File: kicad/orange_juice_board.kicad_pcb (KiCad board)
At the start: 2 copper layers, 85 x 56 mm, 56 parts, among them J10 GPIO12_Head, J10 PWM_OUT1, J11 CONN_UART, J12 Conn_01x08, J12 PWM_OUT2, J13 GPIO6_Head, J14 GPIO11_Head, J15 PWM_OUT3, J2 DC_INPUT, J3 CONN_ADXL345, J4 OrangePi Zero GPIO PINs, J7 OrangePi Zero Function Interf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, J8 FAN_5v, J9 PWR_5v, Q2 AO3400A, Q3 AO3400A, Q4 AO3400A, U1 USBLC6-2SC6, U2 TPS5430DDA, U3 USBLC6-2SC6

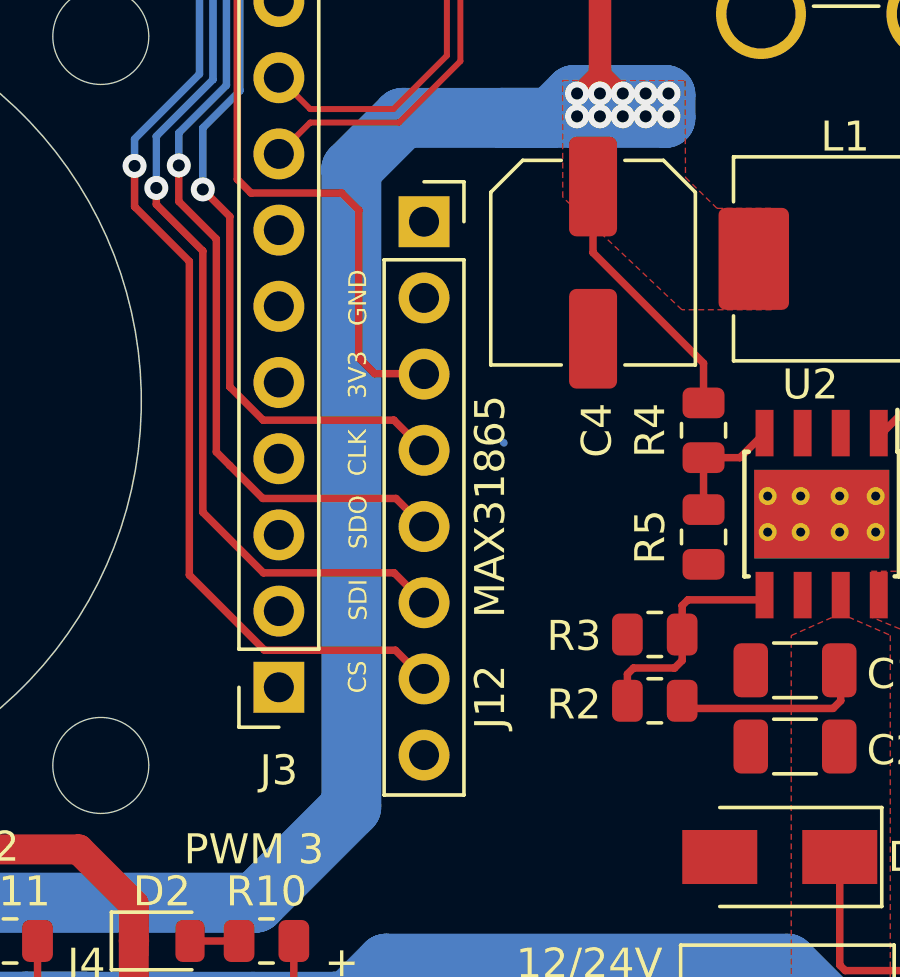
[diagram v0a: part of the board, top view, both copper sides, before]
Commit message: update to v0.7
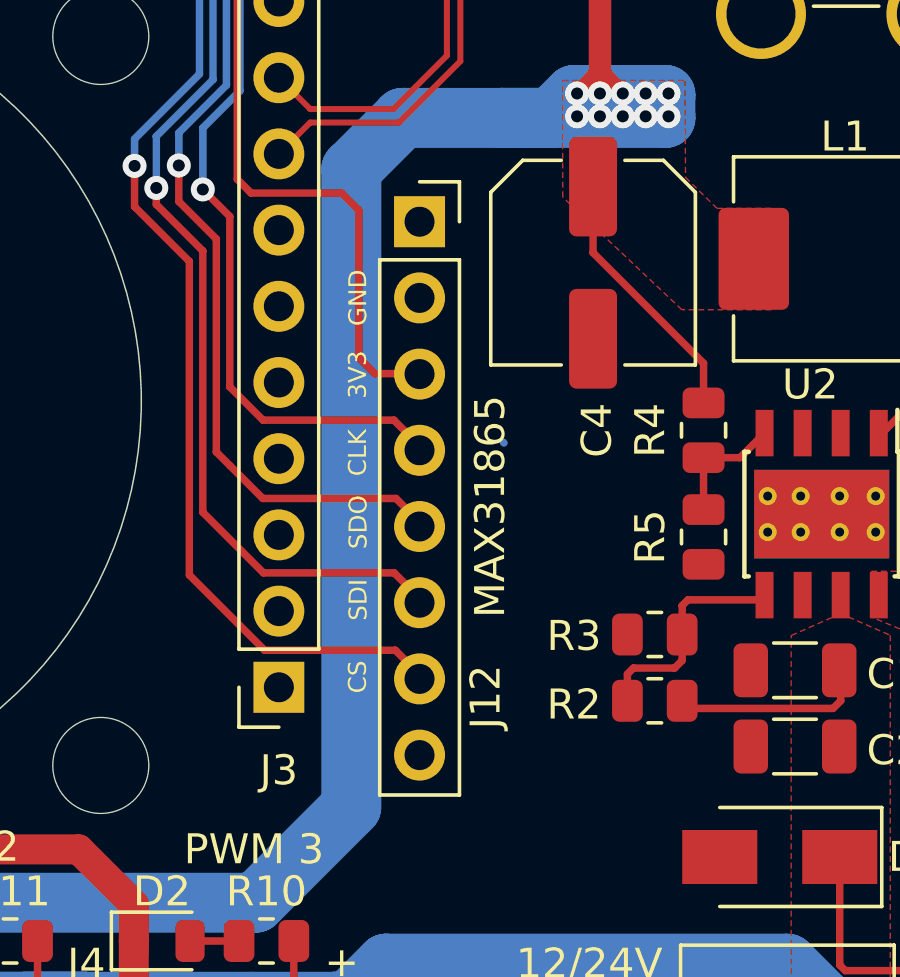
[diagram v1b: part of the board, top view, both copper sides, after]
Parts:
- moved J12 0.15 mm to (148.8, 83.7)
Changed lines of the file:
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@@
     (fp_line (start 3.7 -3.4) (end -3.7 -3.4) (layer "F.SilkS") (width 0.12))
     (fp_line (start 3.7 3.4) (end 3.7 1.9) (layer "F.SilkS") (width 0.12))
+    (fp_line (start 4.45 1.95) (end 4.45 -1.95) (layer "F.CrtYd") (width 0.05))
+    (fp_line (start 3.85 1.95) (end 4.45 1.95) (layer "F.CrtYd") (width 0.05))
+    (fp_line (start 3.85 -3.58) (end -3.85 -3.58) (layer "F.CrtYd") (width 0.05))
+    (fp_line (start -3.85 1.95) (end -3.85 3.58) (layer "F.CrtYd") (width 0.05))
+    (fp_line (start -4.45 1.95) (end -3.85 1.95) (layer "F.CrtYd") (width 0.05))
+    (fp_line (start -4.45 -1.95) (end -4.45 1.95) (layer "F.CrtYd") (width 0.05))
+    (fp_line (start 4.45 -1.95) (end 3.85 -1.95) (layer "F.CrtYd") (width 0.05))
+    (fp_line (start -3.85 -1.95) (end -4.45 -1.95) (layer "F.CrtYd") (width 0.05))
+    (fp_line (start 3.85 3.58) (end 3.85 1.95) (layer "F.CrtYd") (width 0.05))
+    (fp_line (start -3.85 3.58) (end 3.85 3.58) (layer "F.CrtYd") (width 0.05))
     (fp_line (start 3.85 -1.95) (end 3.85 -3.58) (layer "F.CrtYd") (width 0.05))
-    (fp_line (start 3.85 -3.58) (end -3.85 -3.58) (layer "F.CrtYd") (width 0.05))
-    (fp_line (start 4.45 1.95) (end 4.45 -1.95) (layer "F.CrtYd") (width 0.05))
     (fp_line (start -3.85 -3.58) (end -3.85 -1.95) (layer "F.CrtYd") (width 0.05))
-    (fp_line (start -4.45 1.95) (end -3.85 1.95) (layer "F.CrtYd") (width 0.05))
-    (fp_line (start -3.85 3.58) (end 3.85 3.58) (layer "F.CrtYd") (width 0.05))
-    (fp_line (start 3.85 3.58) (end 3.85 1.95) (layer "F.CrtYd") (width 0.05))
-    (fp_line (start -3.85 -1.95) (end -4.45 -1.95) (layer "F.CrtYd") (width 0.05))
-    (fp_line (start 4.45 -1.95) (end 3.85 -1.95) (layer "F.CrtYd") (width 0.05))
-    (fp_line (start -3.85 1.95) (end -3.85 3.58) (layer "F.CrtYd") (width 0.05))
-    (fp_line (start 3.85 1.95) (end 4.45 1.95) (layer "F.CrtYd") (width 0.05))
-    (fp_line (start -4.45 -1.95) (end -4.45 1.95) (layer "F.CrtYd") (width 0.05))
     (fp_line (start 3.6 3.325) (end -3.6 3.325) (layer "F.Fab") (width 0.1))
     (fp_line (start -3.6 3.325) (end -3.6 -3.325) (layer "F.Fab") (width 0.1))
@@
   )
   (footprint "Connector_PinSocket_2.54mm:PinSocket_1x08_P2.54mm_Vertical" locked (layer "F.Cu")
-    (at 148.925 83.725)
+    (at 148.775 83.725)
     (descr "Through hole straight socket strip, 1x08, 2.54mm pitch, single row (from Kicad 4.0.7), script generated")
     (tags "Through hole socket strip THT 1x08 2.54mm single row")
